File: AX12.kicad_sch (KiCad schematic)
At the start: 14 parts, among them J25 Conn_AX12, J29 Conn_AX12, Q10 MMBF170, Q5 MMBF170, Q9 MMBF170, U5 74LVC2G241

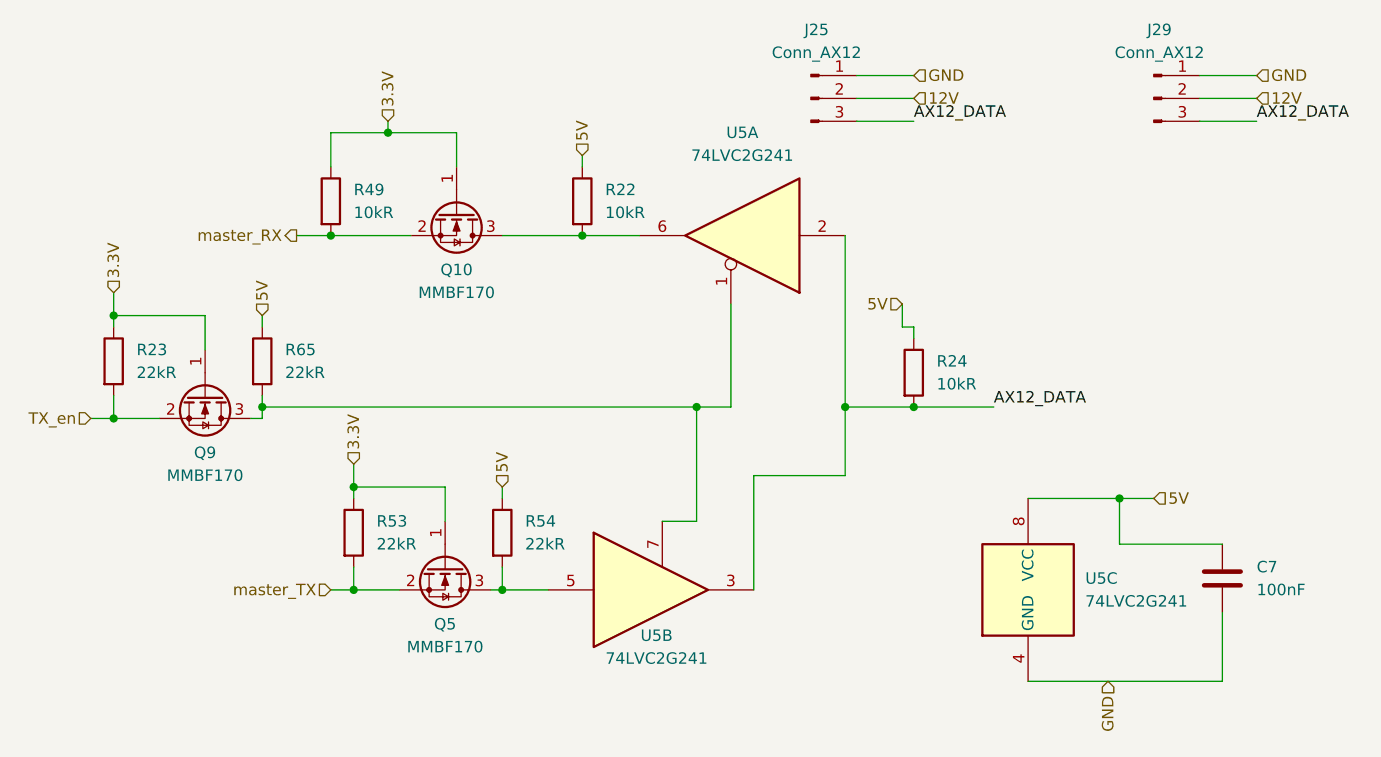
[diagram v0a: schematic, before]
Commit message: update BOM + add big capas (do not take DNP into account)
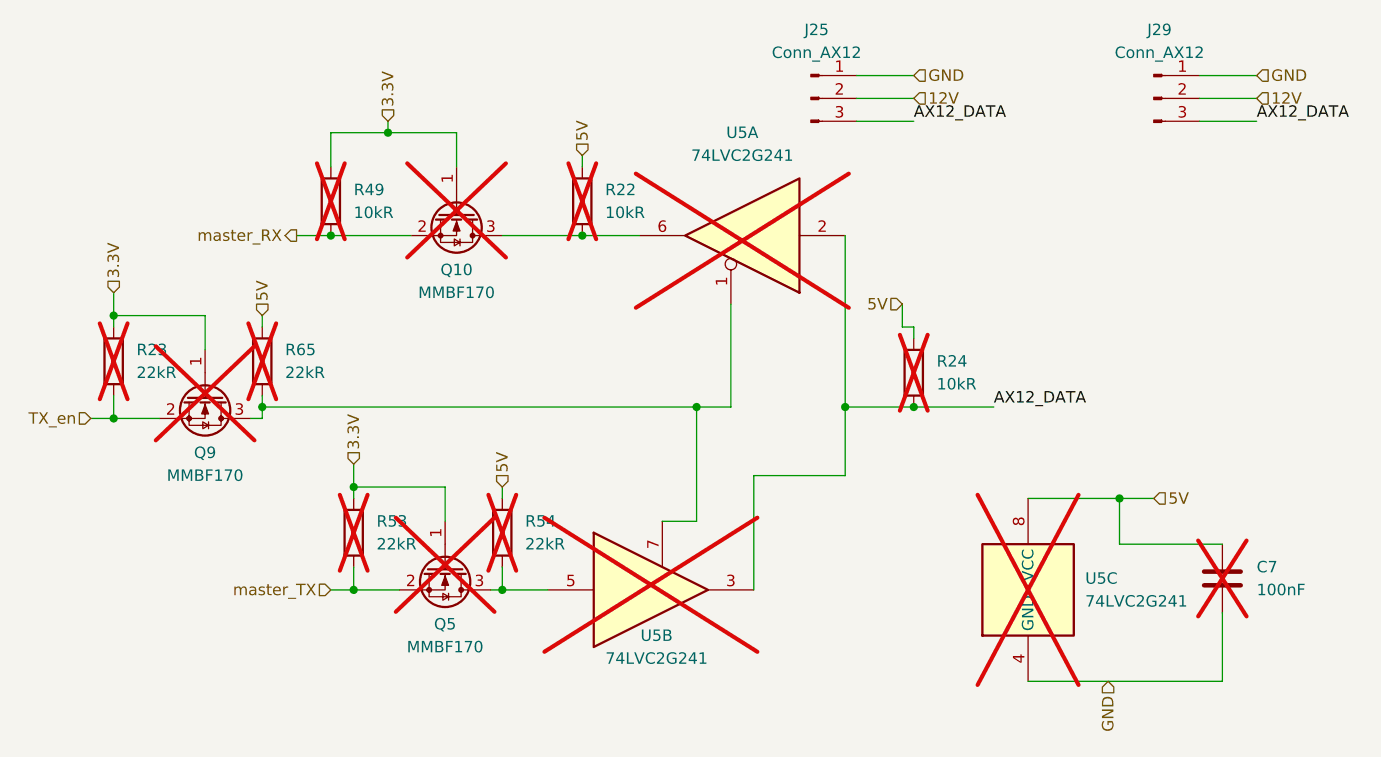
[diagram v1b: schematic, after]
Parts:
- C7, Q10, Q5, Q9, R22, R23, R24, R49, R53, R54, R65, U5: now not fitted
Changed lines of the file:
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@@
 		(in_bom yes)
 		(on_board yes)
-		(dnp no)
+		(dnp yes)
 		(fields_autoplaced yes)
 		(property "Reference" "U5"
@@
 		(in_bom yes)
 		(on_board yes)
-		(dnp no)
+		(dnp yes)
 		(fields_autoplaced yes)
 		(property "Reference" "R23"
@@
 		(in_bom yes)
 		(on_board yes)
-		(dnp no)
+		(dnp yes)
 		(fields_autoplaced yes)
 		(property "Reference" "R22"
@@
 		(in_bom yes)
 		(on_board yes)
-		(dnp no)
+		(dnp yes)
 		(fields_autoplaced yes)
 		(property "Reference" "U5"
@@
 		(in_bom yes)
 		(on_board yes)
-		(dnp no)
+		(dnp yes)
 		(fields_autoplaced yes)
 		(property "Reference" "Q10"
@@
 		(in_bom yes)
 		(on_board yes)
-		(dnp no)
+		(dnp yes)
 		(fields_autoplaced yes)
 		(property "Reference" "R49"
@@
 		(in_bom yes)
 		(on_board yes)
-		(dnp no)
+		(dnp yes)
 		(fields_autoplaced yes)
 		(property "Reference" "Q5"
@@
 		(in_bom yes)
 		(on_board yes)
-		(dnp no)
+		(dnp yes)
 		(fields_autoplaced yes)
 		(property "Reference" "R54"
@@
 		(in_bom yes)
 		(on_board yes)
-		(dnp no)
+		(dnp yes)
 		(fields_autoplaced yes)
 		(property "Reference" "C7"
@@
 		(in_bom yes)
 		(on_board yes)
-		(dnp no)
+		(dnp yes)
 		(fields_autoplaced yes)
 		(property "Reference" "U5"
@@
 		(in_bom yes)
 		(on_board yes)
-		(dnp no)
+		(dnp yes)
 		(fields_autoplaced yes)
 		(property "Reference" "Q9"
@@
 		(in_bom yes)
 		(on_board yes)
-		(dnp no)
+		(dnp yes)
 		(fields_autoplaced yes)
 		(property "Reference" "R65"
@@
 		(in_bom yes)
 		(on_board yes)
-		(dnp no)
+		(dnp yes)
 		(fields_autoplaced yes)
 		(property "Reference" "R24"
@@
 		(in_bom yes)
 		(on_board yes)
-		(dnp no)
+		(dnp yes)
 		(fields_autoplaced yes)
 		(property "Reference" "R53"

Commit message: fix DNP (was just for checking what was to be bought)
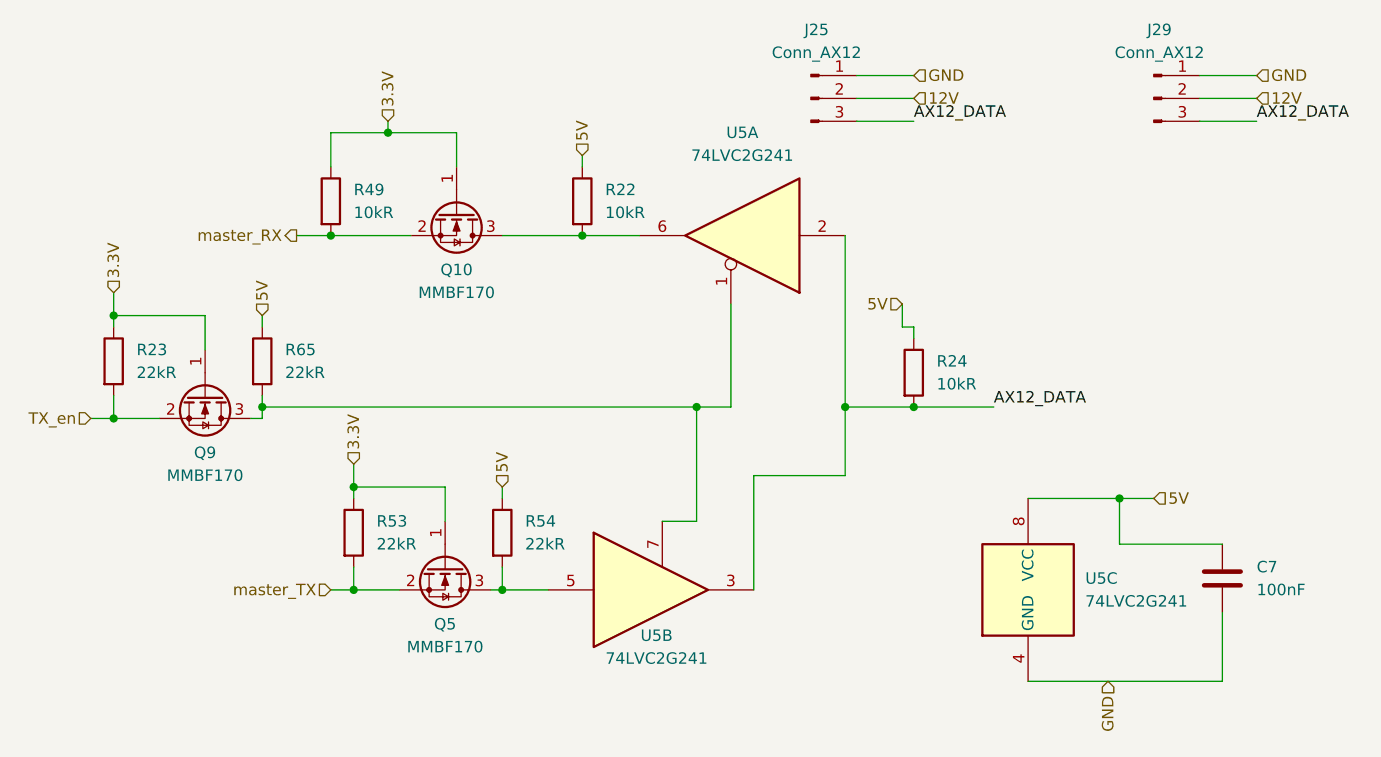
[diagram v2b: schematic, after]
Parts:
- C7, Q10, Q5, Q9, R22, R23, R24, R49, R53, R54, R65, U5: now fitted
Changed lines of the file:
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@@
 		(in_bom yes)
 		(on_board yes)
-		(dnp yes)
+		(dnp no)
 		(fields_autoplaced yes)
 		(property "Reference" "U5"
@@
 		(in_bom yes)
 		(on_board yes)
-		(dnp yes)
+		(dnp no)
 		(fields_autoplaced yes)
 		(property "Reference" "R23"
@@
 		(in_bom yes)
 		(on_board yes)
-		(dnp yes)
+		(dnp no)
 		(fields_autoplaced yes)
 		(property "Reference" "R22"
@@
 		(in_bom yes)
 		(on_board yes)
-		(dnp yes)
+		(dnp no)
 		(fields_autoplaced yes)
 		(property "Reference" "U5"
@@
 		(in_bom yes)
 		(on_board yes)
-		(dnp yes)
+		(dnp no)
 		(fields_autoplaced yes)
 		(property "Reference" "Q10"
@@
 		(in_bom yes)
 		(on_board yes)
-		(dnp yes)
+		(dnp no)
 		(fields_autoplaced yes)
 		(property "Reference" "R49"
@@
 		(in_bom yes)
 		(on_board yes)
-		(dnp yes)
+		(dnp no)
 		(fields_autoplaced yes)
 		(property "Reference" "Q5"
@@
 		(in_bom yes)
 		(on_board yes)
-		(dnp yes)
+		(dnp no)
 		(fields_autoplaced yes)
 		(property "Reference" "R54"
@@
 		(in_bom yes)
 		(on_board yes)
-		(dnp yes)
+		(dnp no)
 		(fields_autoplaced yes)
 		(property "Reference" "C7"
@@
 		(in_bom yes)
 		(on_board yes)
-		(dnp yes)
+		(dnp no)
 		(fields_autoplaced yes)
 		(property "Reference" "U5"
@@
 		(in_bom yes)
 		(on_board yes)
-		(dnp yes)
+		(dnp no)
 		(fields_autoplaced yes)
 		(property "Reference" "Q9"
@@
 		(in_bom yes)
 		(on_board yes)
-		(dnp yes)
+		(dnp no)
 		(fields_autoplaced yes)
 		(property "Reference" "R65"
@@
 		(in_bom yes)
 		(on_board yes)
-		(dnp yes)
+		(dnp no)
 		(fields_autoplaced yes)
 		(property "Reference" "R24"
@@
 		(in_bom yes)
 		(on_board yes)
-		(dnp yes)
+		(dnp no)
 		(fields_autoplaced yes)
 		(property "Reference" "R53"
